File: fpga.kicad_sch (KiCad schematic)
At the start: 2 parts, among them U1 ICE40HX4K-TQ144

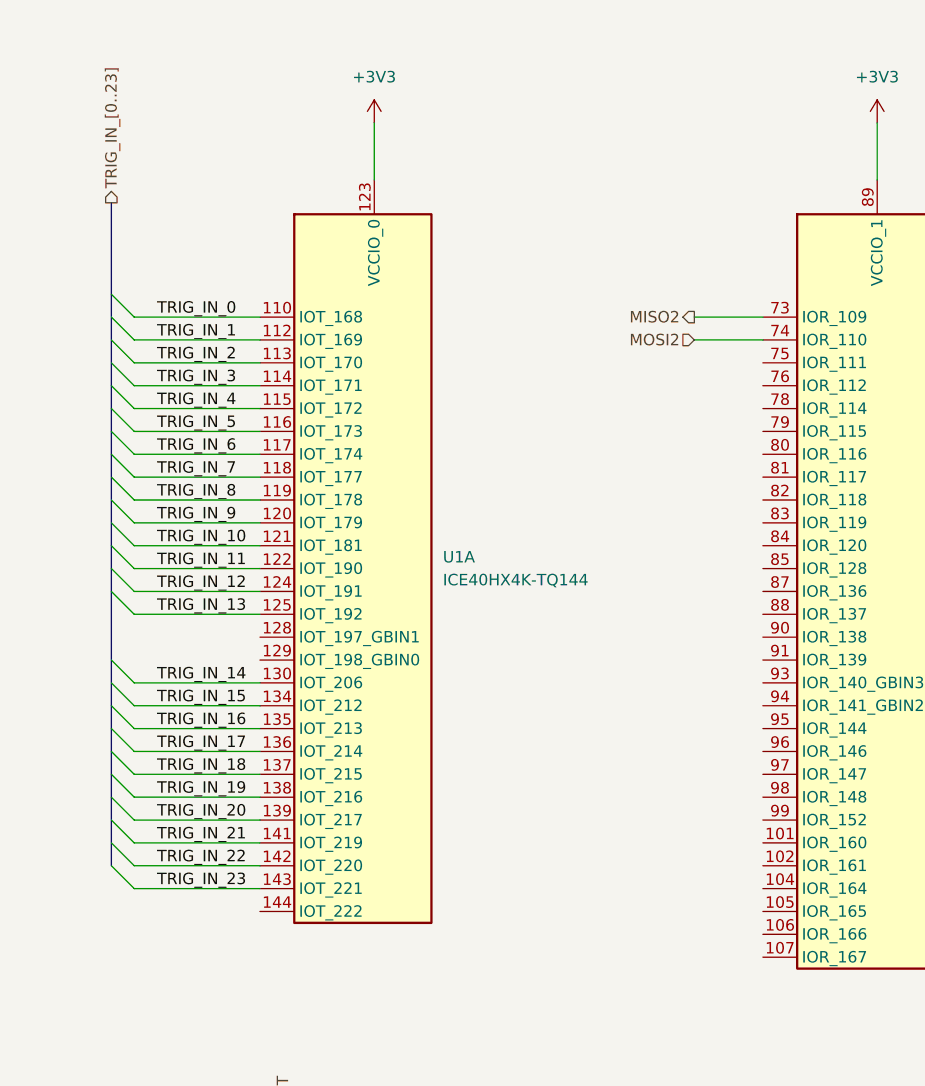
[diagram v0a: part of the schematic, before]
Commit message: cleanup
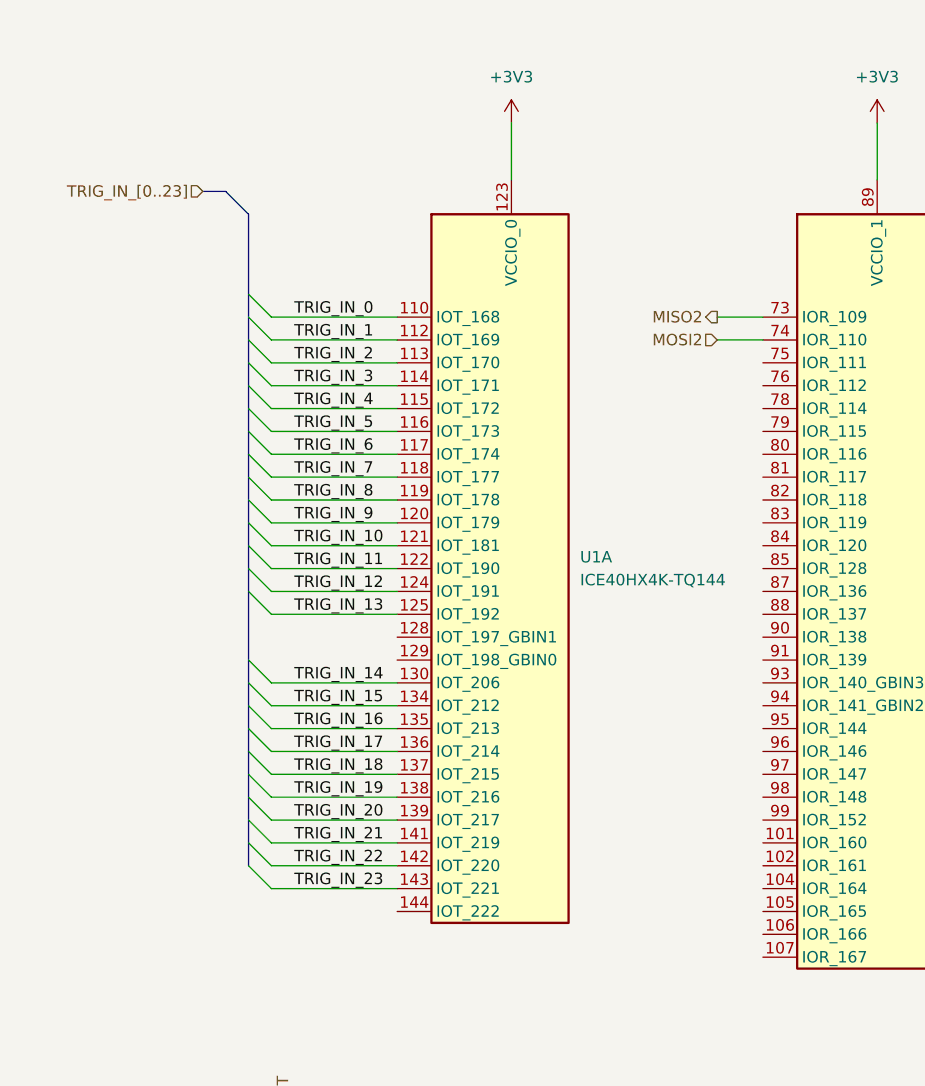
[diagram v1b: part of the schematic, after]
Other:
- moved on the sheet: U1A
